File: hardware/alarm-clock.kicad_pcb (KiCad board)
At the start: 2 copper layers, 68.6 x 86.4 mm, 36 parts, among them CON1 BARREL_JACK, CON2 BARREL_JACK, IC1 ATMEGA328P-PU, P1 PROGRAMMER, Q1 Q_NPN_BCE, Q2 Q_NPN_BCE, SW1 SPST, U1 LM7805CT, U2 DS1307, U3 4Dig7Seg, Y1 38.7kHz, Y2 16MHz

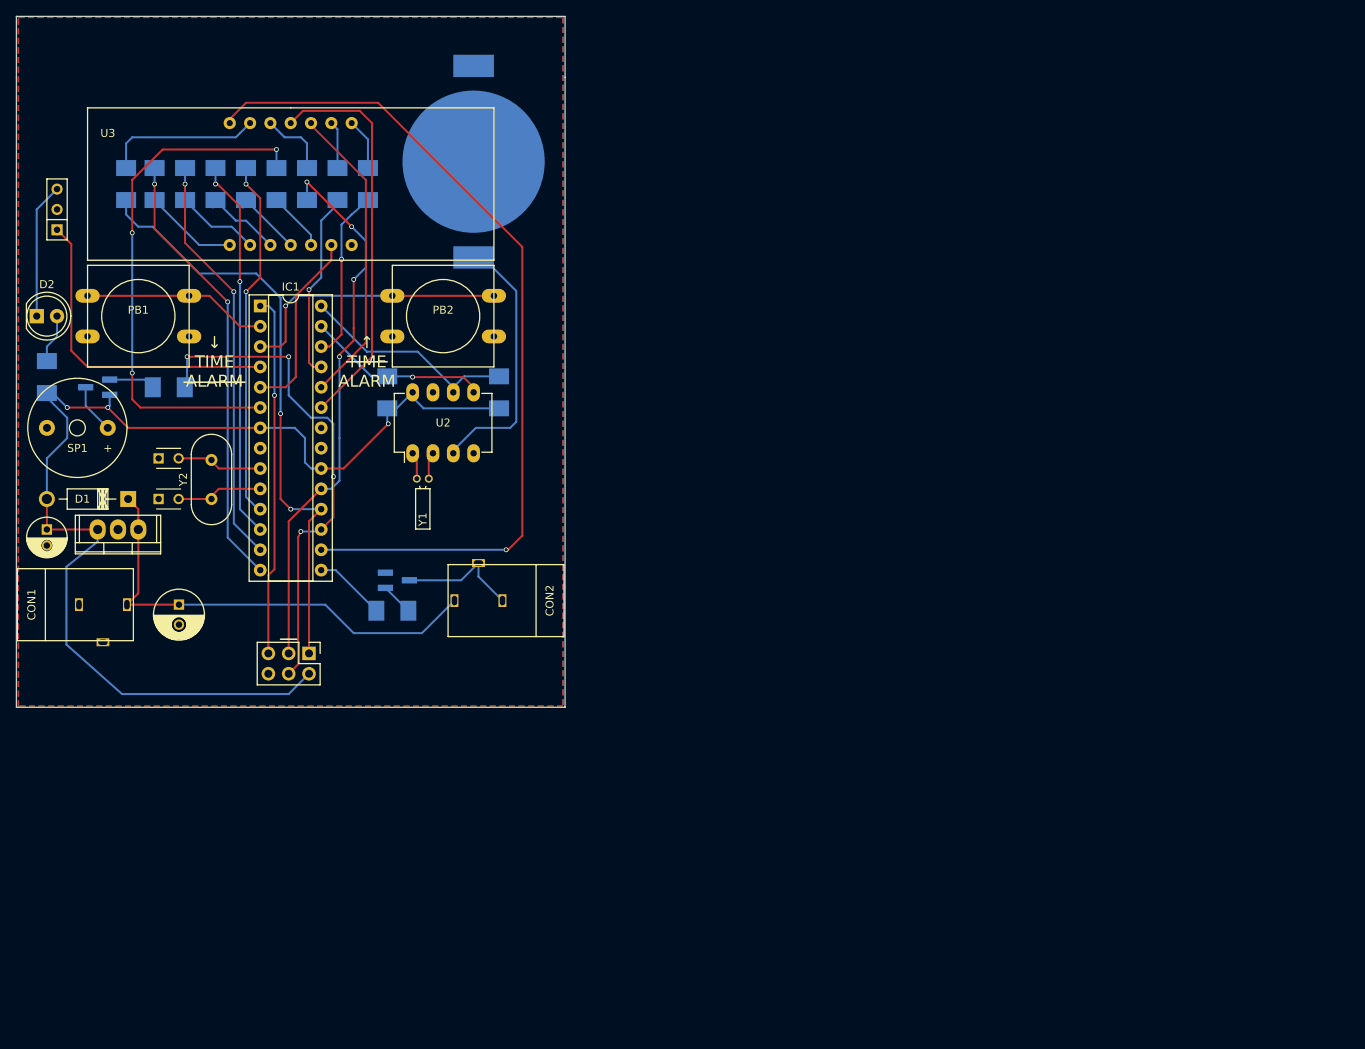
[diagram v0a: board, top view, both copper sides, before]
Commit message: WIP on V3
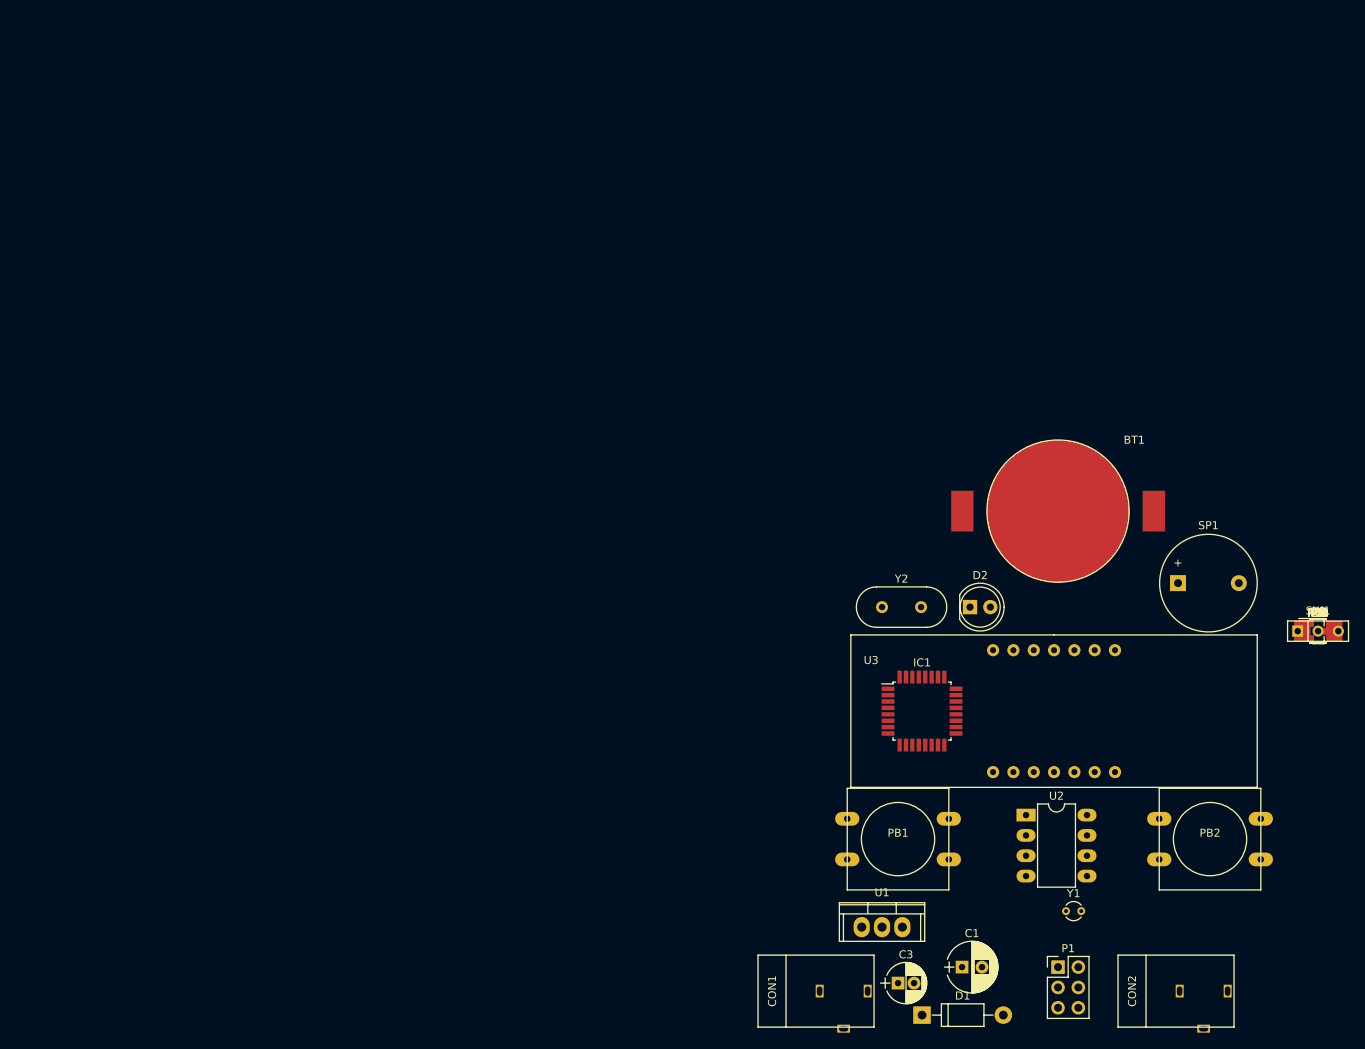
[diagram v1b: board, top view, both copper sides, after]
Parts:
- BT1, Q2, R1, R10, R11, R12, R13, R14, R2, R3, R4, R5, R6, R7, R8, R9: moved to F.Cu
- C1: footprint Capacitors_ThroughHole:C_Radial_D6.3_L11.2_P2.5 -> Capacitors_THT:CP_Radial_D6.3mm_P2.50mm
- C3: footprint Capacitors_ThroughHole:C_Radial_D5_L11_P2 -> Capacitors_THT:CP_Radial_D5.0mm_P2.00mm
- C5, C6: footprint Capacitors_ThroughHole:C_Disc_D3_P2.5 -> Capacitors_SMD:C_1210_HandSoldering
- D1: footprint Diodes_THT:Diode_DO-41_SOD81_Horizontal_RM10 -> Diodes_THT:D_DO-41_SOD81_P10.16mm_Horizontal
- IC1: footprint Housings_DIP:DIP-28_W7.62mm_Socket -> Housings_QFP:TQFP-32_7x7mm_Pitch0.8mm
- Y1: footprint Crystals:Crystal_Round_Horizontal_2mm -> Crystals:Crystal_Round_d2.0mm_Vertical
- moved SW1 166.2 mm to (181.5, 95.0), turned to 0 degrees
- moved R5 162.0 mm to (181.5, 95.0), turned to 0 degrees
- moved R7 159.1 mm to (181.5, 95.0), turned to 0 degrees
- moved R6 155.8 mm to (181.5, 95.0), turned to 0 degrees
- moved Q2 155.6 mm to (181.5, 95.0), turned to 0 degrees
- moved R8 152.3 mm to (181.5, 95.0), turned to 0 degrees
- moved R10 148.7 mm to (181.5, 95.0), turned to 0 degrees
- moved R2 146.9 mm to (181.5, 95.0), turned to 0 degrees
- moved C5 146.5 mm to (181.5, 95.0)
- moved C6 145.9 mm to (181.5, 95.0)
- moved R11 145.2 mm to (181.5, 95.0), turned to 0 degrees
- moved R12 141.7 mm to (181.5, 95.0), turned to 0 degrees
- moved SP1 138.9 mm to (164.0, 89.0), turned to 0 degrees
- moved R9 138.2 mm to (181.5, 95.0), turned to 0 degrees
- moved R13 134.7 mm to (181.5, 95.0), turned to 0 degrees
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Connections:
- IC1 pad 21: (no net) -> Net-(IC1-Pad21)
- U2 pad 7: (no net) -> Net-(U2-Pad7)
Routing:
- net +5V: track 147.3 -> 0.00 mm, vias 3 -> 0
- net PB2: track 107.3 -> 0.00 mm, vias 1 -> 0
- net PB4: track 75.5 -> 0.00 mm, vias 2 -> 0
- net PB5: track 69.0 -> 0.00 mm, vias 4 -> 0
- net PD4: track 65.8 -> 0.00 mm, vias 3 -> 0
- net PB3: track 64.7 -> 0.00 mm, vias 4 -> 0
- net VPP: track 58.6 -> 0.00 mm
- net PB0: track 55.7 -> 0.00 mm, vias 2 -> 0
- net PD7: track 51.6 -> 0.00 mm, vias 2 -> 0
- net PC0: track 50.2 -> 0.00 mm
- net PD6: track 47.6 -> 0.00 mm, vias 2 -> 0
- net RESET: track 45.1 -> 0.00 mm, vias 1 -> 0
- net PD5: track 45.0 -> 0.00 mm, vias 2 -> 0
- net PD2: track 40.9 -> 0.00 mm
- net PC1: track 38.2 -> 0.00 mm
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- removed copper zone on B.Cu, net GND
- removed copper zone on F.Cu, net GND
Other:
- board outline removed
- board text removed: "↑ TIME ALARM"
- board text removed: "↓ TIME ALARM"
